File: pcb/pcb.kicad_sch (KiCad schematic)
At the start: 96 parts, among them J1 OLED, SW1 RotaryEncoder_Switch, U1 Elite-C

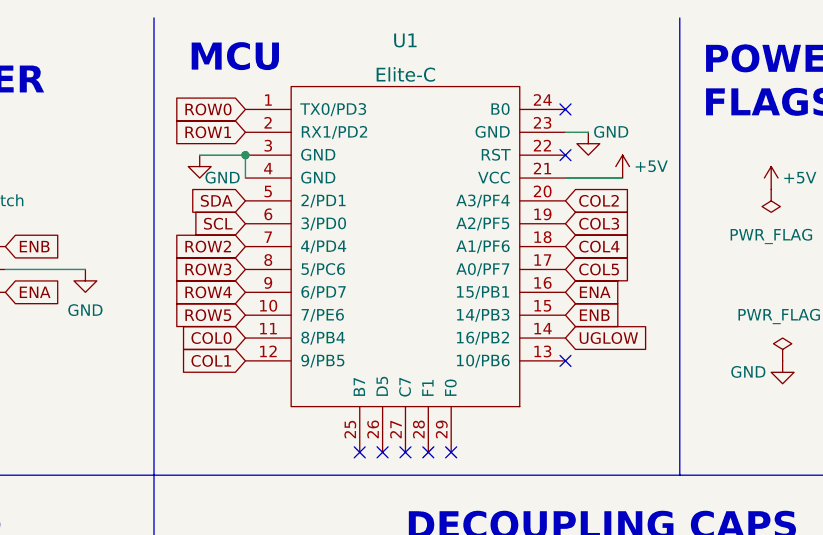
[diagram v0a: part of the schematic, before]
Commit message: Finished routing.
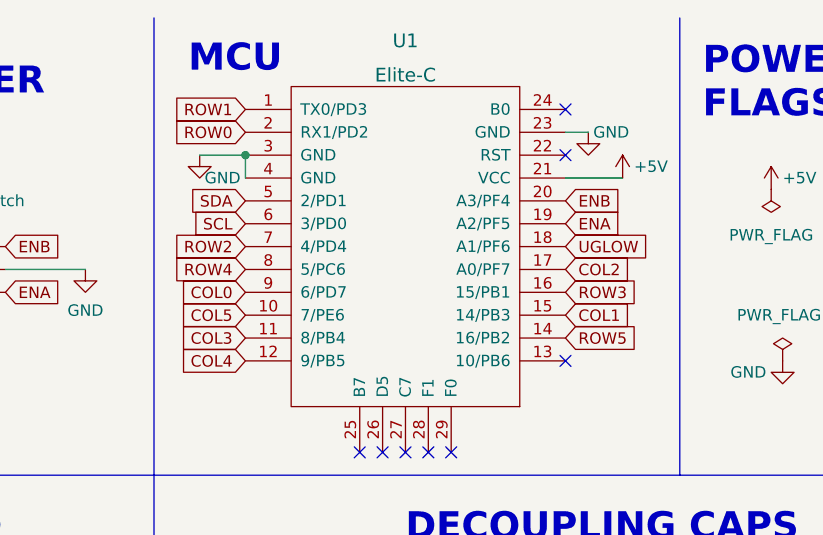
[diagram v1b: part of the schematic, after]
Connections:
- net COL0: now also U1.9 (6/PD7); no longer U1.11 (8/PB4)
- net COL1: now also U1.15 (14/PB3); no longer U1.12 (9/PB5)
- net COL2: now also U1.17 (A0/PF7); no longer U1.20 (A3/PF4)
- net COL3: now also U1.11 (8/PB4); no longer U1.19 (A2/PF5)
- net COL4: now also U1.12 (9/PB5); no longer U1.18 (A1/PF6)
- net COL5: now also U1.10 (7/PE6); no longer U1.17 (A0/PF7)
- net ENA: now also U1.19 (A2/PF5); no longer U1.16 (15/PB1)
- net ENB: now also U1.20 (A3/PF4); no longer U1.15 (14/PB3)
- net ROW0: now also U1.2 (RX1/PD2); no longer U1.1 (TX0/PD3)
- net ROW1: now also U1.1 (TX0/PD3); no longer U1.2 (RX1/PD2)
- net ROW3: now also U1.16 (15/PB1); no longer U1.8 (5/PC6)
- net ROW4: now also U1.8 (5/PC6); no longer U1.9 (6/PD7)
- net ROW5: now also U1.14 (16/PB2); no longer U1.10 (7/PE6)
- net UGLOW: now also U1.18 (A1/PF6); no longer U1.14 (16/PB2)
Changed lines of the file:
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@@
     )
   )
-  (global_label "ROW0" (shape input) (at 179.07 22.86 180) (fields_autoplaced)
+  (global_label "ROW0" (shape input) (at 179.07 25.4 180) (fields_autoplaced)
     (effects (font (size 1.27 1.27)) (justify right))
-    (property "Intersheet References" "${INTERSHEET_REFS}" (id 0) (at 171.3955 22.7806 0)
+    (property "Intersheet References" "${INTERSHEET_REFS}" (id 0) (at 171.3955 25.3206 0)
       (effects (font (size 1.27 1.27)) (justify right) hide)
     )
@@
     )
   )
-  (global_label "ROW4" (shape input) (at 179.07 43.18 180) (fields_autoplaced)
+  (global_label "ROW4" (shape input) (at 179.07 40.64 180) (fields_autoplaced)
     (effects (font (size 1.27 1.27)) (justify right))
-    (property "Intersheet References" "${INTERSHEET_REFS}" (id 0) (at 171.3955 43.1006 0)
+    (property "Intersheet References" "${INTERSHEET_REFS}" (id 0) (at 171.3955 40.5606 0)
       (effects (font (size 1.27 1.27)) (justify right) hide)
     )
   )
-  (global_label "COL1" (shape input) (at 179.07 50.8 180) (fields_autoplaced)
-    (effects (font (size 1.27 1.27)) (justify right))
-    (property "Intersheet References" "${INTERSHEET_REFS}" (id 0) (at 171.8188 50.8794 0)
-      (effects (font (size 1.27 1.27)) (justify right) hide)
+  (global_label "COL1" (shape input) (at 214.63 45.72 0) (fields_autoplaced)
+    (effects (font (size 1.27 1.27)) (justify left))
+    (property "Intersheet References" "${INTERSHEET_REFS}" (id 0) (at 221.8812 45.6406 0)
+      (effects (font (size 1.27 1.27)) (justify left) hide)
     )
   )
-  (global_label "COL3" (shape input) (at 214.63 35.56 0) (fields_autoplaced)
-    (effects (font (size 1.27 1.27)) (justify left))
-    (property "Intersheet References" "${INTERSHEET_REFS}" (id 0) (at 221.8812 35.4806 0)
-      (effects (font (size 1.27 1.27)) (justify left) hide)
+  (global_label "COL3" (shape input) (at 179.07 48.26 180) (fields_autoplaced)
+    (effects (font (size 1.27 1.27)) (justify right))
+    (property "Intersheet References" "${INTERSHEET_REFS}" (id 0) (at 171.8188 48.3394 0)
+      (effects (font (size 1.27 1.27)) (justify right) hide)
     )
   )
@@
     )
   )
-  (global_label "ENA" (shape input) (at 214.63 43.18 0) (fields_autoplaced)
+  (global_label "ENA" (shape input) (at 214.63 35.56 0) (fields_autoplaced)
     (effects (font (size 1.27 1.27)) (justify left))
-    (property "Intersheet References" "${INTERSHEET_REFS}" (id 0) (at 220.6112 43.1006 0)
+    (property "Intersheet References" "${INTERSHEET_REFS}" (id 0) (at 220.6112 35.4806 0)
       (effects (font (size 1.27 1.27)) (justify left) hide)
     )
   )
-  (global_label "COL5" (shape input) (at 214.63 40.64 0) (fields_autoplaced)
-    (effects (font (size 1.27 1.27)) (justify left))
-    (property "Intersheet References" "${INTERSHEET_REFS}" (id 0) (at 221.8812 40.5606 0)
-      (effects (font (size 1.27 1.27)) (justify left) hide)
+  (global_label "COL5" (shape input) (at 179.07 45.72 180) (fields_autoplaced)
+    (effects (font (size 1.27 1.27)) (justify right))
+    (property "Intersheet References" "${INTERSHEET_REFS}" (id 0) (at 171.8188 45.7994 0)
+      (effects (font (size 1.27 1.27)) (justify right) hide)
     )
   )
@@
     )
   )
-  (global_label "ROW5" (shape input) (at 179.07 45.72 180) (fields_autoplaced)
-    (effects (font (size 1.27 1.27)) (justify right))
-    (property "Intersheet References" "${INTERSHEET_REFS}" (id 0) (at 171.3955 45.6406 0)
-      (effects (font (size 1.27 1.27)) (justify right) hide)
+  (global_label "ROW5" (shape input) (at 214.63 48.26 0) (fields_autoplaced)
+    (effects (font (size 1.27 1.27)) (justify left))
+    (property "Intersheet References" "${INTERSHEET_REFS}" (id 0) (at 222.3045 48.3394 0)
+      (effects (font (size 1.27 1.27)) (justify left) hide)
     )
   )
-  (global_label "ROW3" (shape input) (at 179.07 40.64 180) (fields_autoplaced)
-    (effects (font (size 1.27 1.27)) (justify right))
-    (property "Intersheet References" "${INTERSHEET_REFS}" (id 0) (at 171.3955 40.5606 0)
-      (effects (font (size 1.27 1.27)) (justify right) hide)
+  (global_label "ROW3" (shape input) (at 214.63 43.18 0) (fields_autoplaced)
+    (effects (font (size 1.27 1.27)) (justify left))
+    (property "Intersheet References" "${INTERSHEET_REFS}" (id 0) (at 222.3045 43.2594 0)
+      (effects (font (size 1.27 1.27)) (justify left) hide)
     )
   )
@@
     )
   )
-  (global_label "ROW1" (shape input) (at 179.07 25.4 180) (fields_autoplaced)
+  (global_label "ROW1" (shape input) (at 179.07 22.86 180) (fields_autoplaced)
     (effects (font (size 1.27 1.27)) (justify right))
-    (property "Intersheet References" "${INTERSHEET_REFS}" (id 0) (at 171.3955 25.3206 0)
+    (property "Intersheet References" "${INTERSHEET_REFS}" (id 0) (at 171.3955 22.7806 0)
       (effects (font (size 1.27 1.27)) (justify right) hide)
     )
@@
     )
   )
-  (global_label "ENB" (shape input) (at 214.63 45.72 0) (fields_autoplaced)
+  (global_label "ENB" (shape input) (at 214.63 33.02 0) (fields_autoplaced)
     (effects (font (size 1.27 1.27)) (justify left))
-    (property "Intersheet References" "${INTERSHEET_REFS}" (id 0) (at 220.7926 45.6406 0)
+    (property "Intersheet References" "${INTERSHEET_REFS}" (id 0) (at 220.7926 32.9406 0)
       (effects (font (size 1.27 1.27)) (justify left) hide)
     )
@@
     )
   )
-  (global_label "UGLOW" (shape input) (at 214.63 48.26 0) (fields_autoplaced)
+  (global_label "UGLOW" (shape input) (at 214.63 38.1 0) (fields_autoplaced)
     (effects (font (size 1.27 1.27)) (justify left))
-    (property "Intersheet References" "${INTERSHEET_REFS}" (id 0) (at 223.4536 48.3394 0)
+    (property "Intersheet References" "${INTERSHEET_REFS}" (id 0) (at 223.4536 38.1794 0)
       (effects (font (size 1.27 1.27)) (justify left) hide)
     )
   )
-  (global_label "COL0" (shape input) (at 179.07 48.26 180) (fields_autoplaced)
+  (global_label "COL0" (shape input) (at 179.07 43.18 180) (fields_autoplaced)
     (effects (font (size 1.27 1.27)) (justify right))
-    (property "Intersheet References" "${INTERSHEET_REFS}" (id 0) (at 171.8188 48.3394 0)
+    (property "Intersheet References" "${INTERSHEET_REFS}" (id 0) (at 171.8188 43.2594 0)
       (effects (font (size 1.27 1.27)) (justify right) hide)
     )
   )
-  (global_label "COL2" (shape input) (at 214.63 33.02 0) (fields_autoplaced)
+  (global_label "COL2" (shape input) (at 214.63 40.64 0) (fields_autoplaced)
     (effects (font (size 1.27 1.27)) (justify left))
-    (property "Intersheet References" "${INTERSHEET_REFS}" (id 0) (at 221.8812 32.9406 0)
+    (property "Intersheet References" "${INTERSHEET_REFS}" (id 0) (at 221.8812 40.5606 0)
       (effects (font (size 1.27 1.27)) (justify left) hide)
     )
@@
     )
   )
-  (global_label "COL4" (shape input) (at 214.63 38.1 0) (fields_autoplaced)
-    (effects (font (size 1.27 1.27)) (justify left))
-    (property "Intersheet References" "${INTERSHEET_REFS}" (id 0) (at 221.8812 38.0206 0)
-      (effects (font (size 1.27 1.27)) (justify left) hide)
+  (global_label "COL4" (shape input) (at 179.07 50.8 180) (fields_autoplaced)
+    (effects (font (size 1.27 1.27)) (justify right))
+    (property "Intersheet References" "${INTERSHEET_REFS}" (id 0) (at 171.8188 50.8794 0)
+      (effects (font (size 1.27 1.27)) (justify right) hide)
     )
   )
